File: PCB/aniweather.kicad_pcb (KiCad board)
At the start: 2 copper layers, 55 x 75 mm, 37 parts, among them SW2 SW_Push, SW3 SW_Push, SW4 SW_DIP_x01, U4 TPS2116DRL, U5 TPS63001

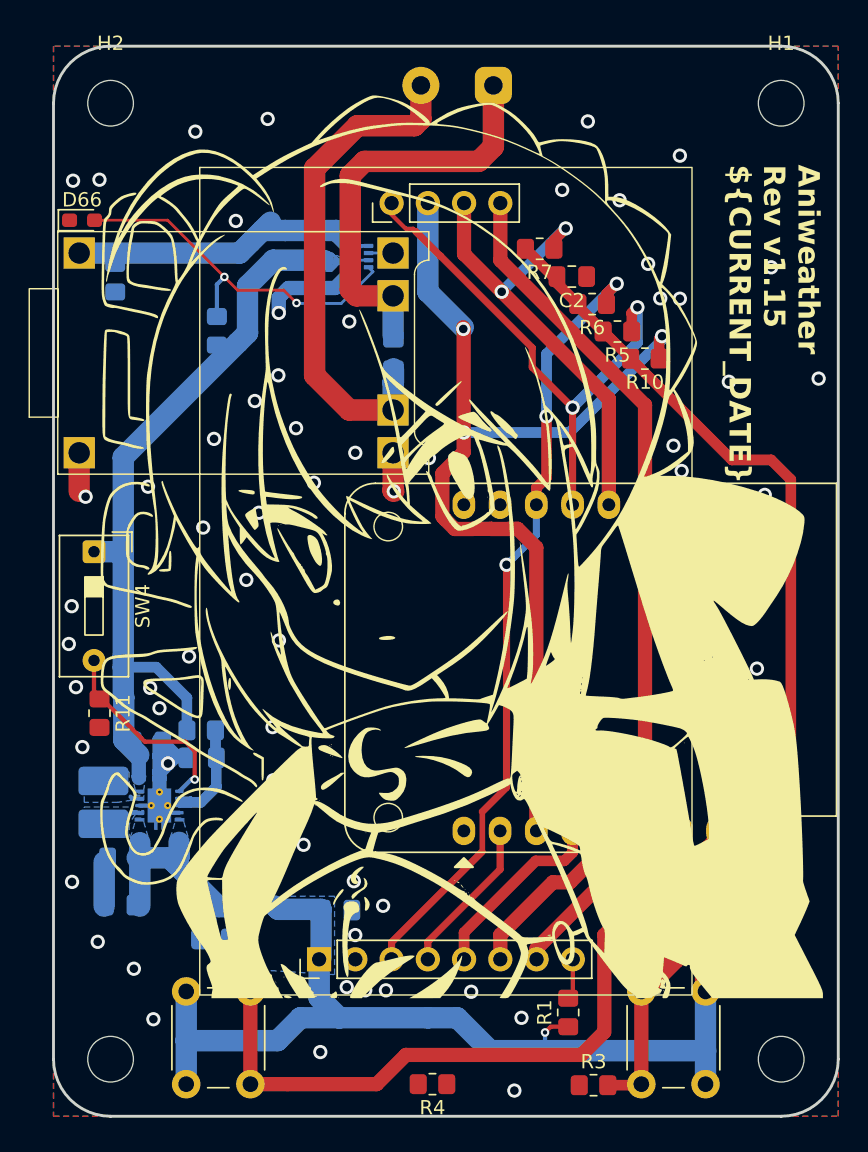
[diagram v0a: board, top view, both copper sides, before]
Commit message: Final revision
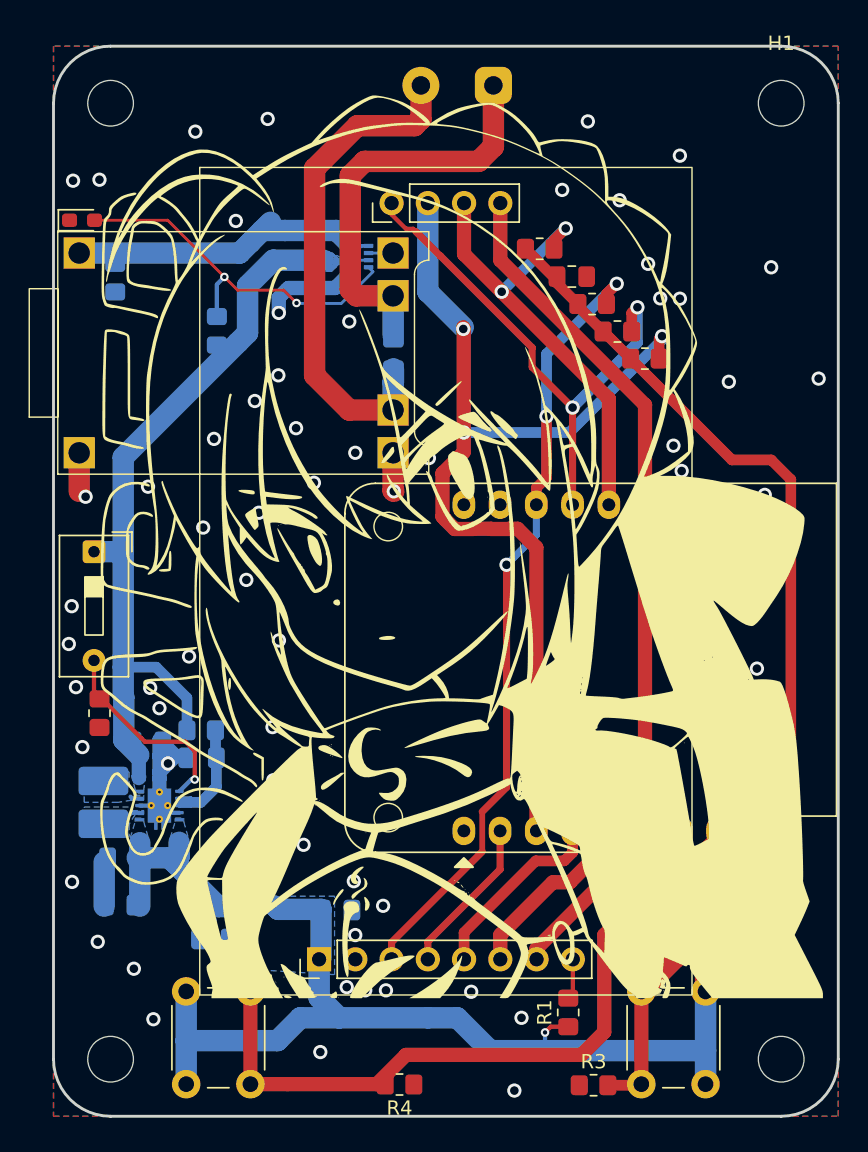
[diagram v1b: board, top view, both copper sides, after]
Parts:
- moved R4 2.31 mm to (136.9, 136.2)
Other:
- board text removed: "${TITLE} Rev ${REVISION} ${CURRENT_DATE}"
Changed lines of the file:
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@@
 		(title "Aniweather")
 		(date "2024-12-06")
-		(rev "v1.15")
+		(rev "v1.16")
 		(company "Cyao")
 		(comment 1 "Anime weather station")
@@
 			(at 0 -1.65 0)
 			(layer "F.SilkS")
+			(hide yes)
 			(effects
 				(font
@@
 			(at 0 -1.65 0)
 			(layer "F.SilkS")
+			(hide yes)
 			(effects
 				(font
@@
 			(at 0 -1.65 90)
 			(layer "F.SilkS")
+			(hide yes)
 			(effects
 				(font
@@
 			(at 0 -1.43 180)
 			(layer "F.SilkS")
+			(hide yes)
 			(effects
 				(font
@@
 			(layer "F.SilkS")
 		)
-		(fp_text user "${REFERENCE}"
-			(at 0 2.5 90)
-			(unlocked yes)
-			(layer "F.Fab")
-			(effects
-				(font
-					(size 1 1)
-					(thickness 0.15)
-				)
-			)
-		)
 		(pad "0" thru_hole rect
 			(at 4 10.5 180)
@@
 			(at 0 -1.68 0)
 			(layer "F.SilkS")
+			(hide yes)
 			(effects
 				(font
@@
 			(at 0 -1.65 0)
 			(layer "F.SilkS")
+			(hide yes)
 			(effects
 				(font
@@
 	(footprint "Resistor_SMD:R_0805_2012Metric_Pad1.20x1.40mm_HandSolder"
 		(layer "F.Cu")
-		(at 139.26 136.175 180)
+		(at 136.95 136.2 180)
 		(descr "Resistor SMD 0805 (2012 Metric), square (rectangular) end terminal, IPC_7351 nominal with elongated pad for handsoldering. (Body size source: IPC-SM-782 page 72, https://www.pcb-3d.com/wordpress/wp-content/uploads/ipc-sm-782a_amendment_1_and_2.pdf), generated with kicad-footprint-generator")
 		(tags "resistor handsolder")
@@
 			(at 3.81 -3.42 90)
 			(layer "F.SilkS")
+			(hide yes)
 			(effects
 				(font
@@
 			(at 0 -4.2 0)
 			(layer "F.SilkS")
+			(hide yes)
 			(effects
 				(font
@@
 			(at 0 -1.65 0)
 			(layer "F.SilkS")
+			(hide yes)
 			(effects
 				(font
@@
 			(at 0 1.68 90)
 			(layer "B.SilkS")
+			(hide yes)
 			(effects
 				(font
@@
 		(attr smd)
 		(fp_line
-			(start -0.261252 0.735)
-			(end 0.261252 0.735)
-			(stroke
-				(width 0.12)
-				(type solid)
-			)
-			(layer "B.SilkS")
-		)
-		(fp_line
-			(start -0.261252 -0.735)
-			(end 0.261252 -0.735)
-			(stroke
-				(width 0.12)
-				(type solid)
-			)
-			(layer "B.SilkS")
-		)
-		(fp_line
 			(start -1.88 0.98)
 			(end 1.88 0.98)
@@
 			(unlocked yes)
 			(layer "B.SilkS")
+			(hide yes)
 			(effects
 				(font
@@
 		(attr exclude_from_pos_files)
 		(fp_line
-			(start 6.6 -1.5)
-			(end 6.6 1.5)
-			(stroke
-				(width 0.12)
-				(type solid)
-			)
-			(layer "B.SilkS")
-		)
-		(fp_line
-			(start 6.6 -1.5)
-			(end -1.5 -1.5)
-			(stroke
-				(width 0.12)
-				(type solid)
-			)
-			(layer "B.SilkS")
-		)
-		(fp_line
-			(start -1.5 1.5)
-			(end 6.6 1.5)
-			(stroke
-				(width 0.12)
-				(type solid)
-			)
-			(layer "B.SilkS")
-		)
-		(fp_line
-			(start -1.5 1.5)
-			(end -1.5 -1.5)
-			(stroke
-				(width 0.12)
-				(type solid)
-			)
-			(layer "B.SilkS")
-		)
-		(fp_line
 			(start 6.88 -1.8)
 			(end 6.88 1.8)
@@
 			(at 2.875 0.375 90)
 			(layer "B.SilkS")
+			(hide yes)
 			(effects
 				(font
@@
 			(unlocked yes)
 			(layer "B.SilkS")
+			(hide yes)
 			(effects
 				(font
@@
 		(sheetfile "aniweather.kicad_sch")
 		(attr smd)
-		(fp_line
-			(start 0.65 -1.16)
-			(end -0.65 -1.16)
-			(stroke
-				(width 0.12)
-				(type default)
-			)
-			(layer "B.SilkS")
-		)
-		(fp_line
-			(start 0.65 1.16)
-			(end -0.4 1.16)
-			(stroke
-				(width 0.12)
-				(type default)
-			)
-			(layer "B.SilkS")
-		)
 		(fp_poly
 			(pts
@@
 			(at 0 1.65 90)
 			(layer "B.SilkS")
+			(hide yes)
 			(effects
 				(font
@@
 			(at 0 1.68 180)
 			(layer "B.SilkS")
+			(hide yes)
 			(effects
 				(font
@@
 			(at 0 1.65 90)
 			(layer "B.SilkS")
+			(hide yes)
 			(effects
 				(font
@@
 			(at 0 1.68 180)
 			(layer "B.SilkS")
+			(hide yes)
 			(effects
 				(font
@@
 			(at 0 1.68 0)
 			(layer "B.SilkS")
+			(hide yes)
 			(effects
 				(font
@@
 		(attr smd)
 		(fp_line
-			(start -0.261252 0.735)
-			(end 0.261252 0.735)
-			(stroke
-				(width 0.12)
-				(type solid)
-			)
-			(layer "B.SilkS")
-		)
-		(fp_line
-			(start -0.261252 -0.735)
-			(end 0.261252 -0.735)
-			(stroke
-				(width 0.12)
-				(type solid)
-			)
-			(layer "B.SilkS")
-		)
-		(fp_line
 			(start 1.88 0.98)
 			(end 1.88 -0.98)
@@
 		(layer "Edge.Cuts")
 	)
-	(gr_text "${TITLE} \nRev ${REVISION} \n${CURRENT_DATE}"
-		(at 159.9 71.725 -90)
-		(layer "F.SilkS")
-		(effects
-			(font
-				(size 1.5 1.5)
-				(thickness 0.3)
-				(bold yes)
-			)
-			(justify left bottom)
-		)
-	)
 	(dimension
